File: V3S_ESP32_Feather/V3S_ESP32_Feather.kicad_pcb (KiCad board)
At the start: 4 copper layers, 30.5 x 48.3 mm, 100 parts, among them J1 USB_B_Micro, J2 Bat, J3 CAM, J4 PWM, J5 U.FL-R-SMT(01), J6 UART, J7 Micro_SD_Card_Det, J8 I2C, J9 I2C, Q1 S8050(SOT-23), U1 V3S, U2 MIC5504-1.2YM5, U3 MIC5501-3.0YM5, U4 ICM-20948, U5 ESP32-PICO-D4, U6 LT1963AxST-3.3, U7 BMP280, U8 MIC5504-1.8YM5, U9 MAX13030EEBET, Y1 X1E0000210832, Y2 CC5V-T1A 32.768KHZ +-20PPM 12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

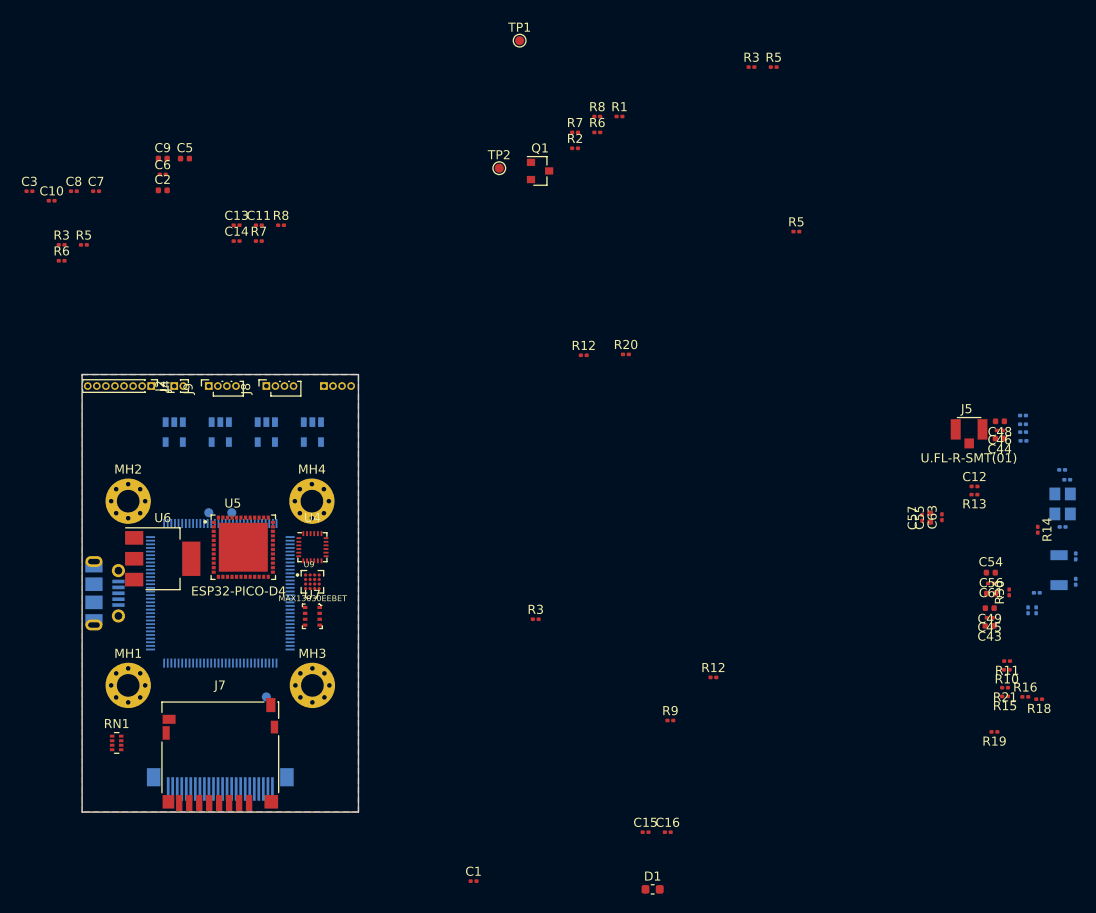
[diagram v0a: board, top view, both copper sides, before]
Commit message: New component placement, progress on rooting
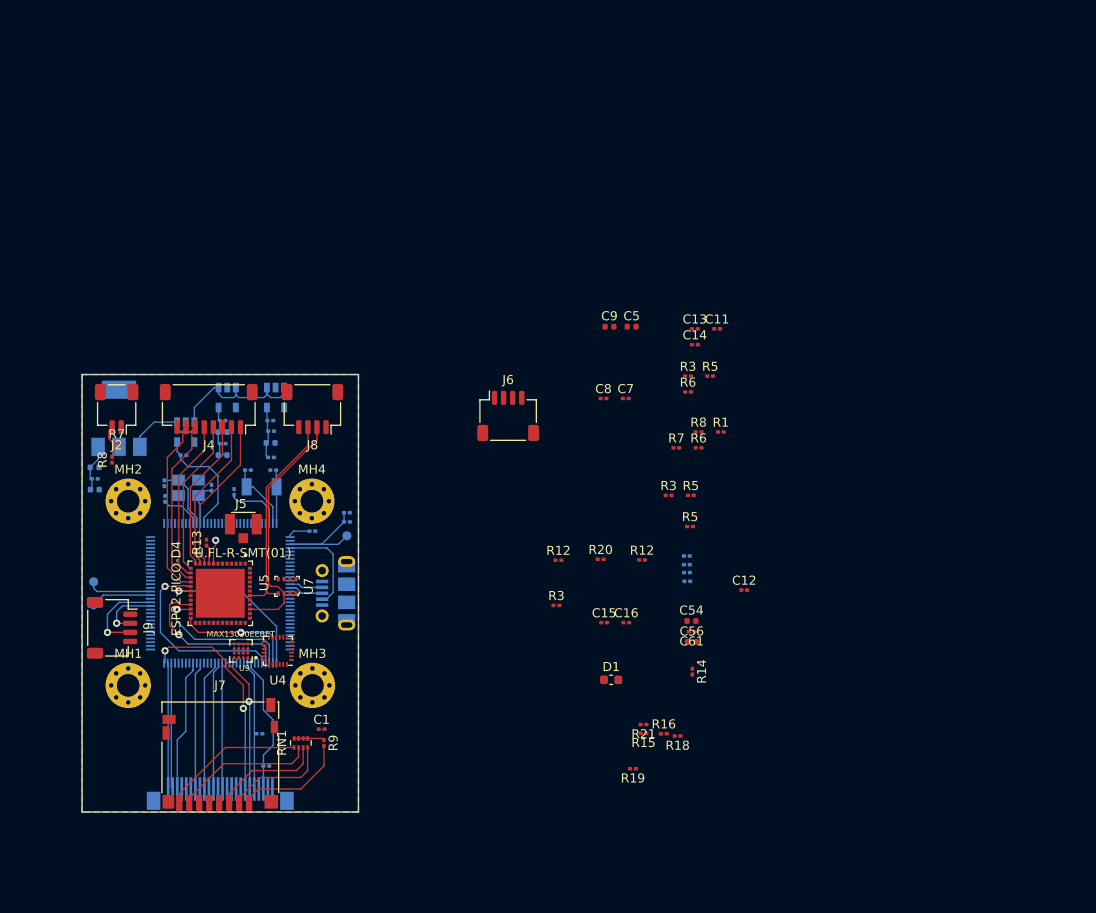
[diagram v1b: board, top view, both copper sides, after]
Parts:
- removed C2: 10uF, Capacitor_SMD:C_0402_1005Metric
- removed Q1: S8050(SOT-23), Package_TO_SOT_SMD:SOT-23
- removed R2: 100K, Resistor_SMD:R_0201_0603Metric
- removed TP1: PWR_SRC, TestPoint:TestPoint_Pad_D1.0mm
- removed the TP2 at (68.9, -2.44)
- removed the U2 at (48.3, 26.7)
- C10, C3, C43, C44, C45, C46, C48, C49, C55, C57, C6, C63, R10, R11, R30, U6: moved to B.Cu
- J2: footprint Connector_PinHeader_1.00mm:PinHeader_1x02_P1.00mm_Vertical -> Connector_JST:JST_SH_SM02B-SRSS-TB_1x02-1MP_P1.00mm_Horizontal
- J4: footprint Connector_PinHeader_1.00mm:PinHeader_1x08_P1.00mm_Vertical -> Connector_JST:JST_SH_SM08B-SRSS-TB_1x08-1MP_P1.00mm_Horizontal
- J6: footprint Connector_PinHeader_1.00mm:PinHeader_1x04_P1.00mm_Vertical -> Connector_JST:JST_SH_SM04B-SRSS-TB_1x04-1MP_P1.00mm_Horizontal; moved to F.Cu
- J8, J9: footprint Connector_PinSocket_1.00mm:PinSocket_1x04_P1.00mm_Vertical -> Connector_JST:JST_SH_SM04B-SRSS-TB_1x04-1MP_P1.00mm_Horizontal
- moved C48 100.0 mm to (24.2, 30.6), turned to 0 degrees
- moved C44 100.0 mm to (24.3, 33.0), turned to 0 degrees
- moved C46 100.0 mm to (24.3, 31.8), turned to 0 degrees
- moved C37 99.6 mm to (31.9, 32.3), turned to 270 degrees
- moved R4 99.0 mm to (32.0, 34.0), turned to 90 degrees
- moved Y1 96.4 mm to (34.6, 32.8), turned to 0 degrees
- moved C36 94.0 mm to (37.1, 32.8), turned to 90 degrees
- moved C41 91.8 mm to (41.1, 30.9), turned to 180 degrees
- moved C40 89.4 mm to (43.9, 30.9), turned to 0 degrees
- moved Y2 88.4 mm to (42.7, 32.7), turned to 270 degrees
- moved C49 86.8 mm to (38.4, 26.7), turned to 0 degrees
- moved C45 86.8 mm to (38.4, 27.9), turned to 0 degrees
- moved C43 86.7 mm to (38.4, 29.2), turned to 0 degrees
- moved R30 86.2 mm to (39.6, 33.3), turned to 270 degrees
- moved R13 84.9 mm to (36.6, 38.9), turned to 90 degrees
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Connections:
- C5 pad 1: /PMIC Power Battery/VIN -> +BATT
- D1 pad 1: /PMIC Power Battery/VIN -> +BATT
- J3 pad 1: (no net) -> /All V3s input output/STROBE
- J3 pad 10: (no net) -> Net-(J3-Pad10)
- J4 pad 1: GND -> /IO34
- J4 pad 2: /IO34 -> /IO35
- J4 pad 3: /IO33 -> /IO32
- J4 pad 4: /IO32 -> /IO33
- J4 pad 5: /IO27 -> /IO25
- J4 pad 7: /IO25 -> /IO27
- J6 pad 3: (no net) -> /TX
- J7 pad 10: (no net) -> Net-(J7-Pad10)
- J7 pad 9: (no net) -> Net-(J7-Pad9)
- R1 pad 1: VBUS -> Net-(D1-Pad2)
- R1 pad 2: Net-(D1-Pad2) -> VBUS
- RN1 pad 1: /All V3s input output/PF4 -> /All V3s input output/PF0
- RN1 pad 2: /All V3s input output/PF3 -> /All V3s input output/PF1
- RN1 pad 3: /All V3s input output/PF1 -> /All V3s input output/PF3
- RN1 pad 4: /All V3s input output/PF0 -> /All V3s input output/PF4
- U1 pad 10: (no net) -> Net-(U1-Pad10)
- U1 pad 11: (no net) -> Net-(U1-Pad11)
- U1 pad 112: (no net) -> Net-(U1-Pad112)
- U1 pad 113: (no net) -> Net-(U1-Pad113)
- U1 pad 114: (no net) -> Net-(U1-Pad114)
- U1 pad 120: (no net) -> Net-(U1-Pad120)
- U1 pad 121: (no net) -> Net-(U1-Pad121)
- U1 pad 124: (no net) -> Net-(U1-Pad124)
- U1 pad 125: (no net) -> Net-(U1-Pad125)
- U1 pad 13: (no net) -> Net-(U1-Pad13)
- U1 pad 14: (no net) -> Net-(U1-Pad14)
- U1 pad 43: (no net) -> Net-(U1-Pad43)
- U1 pad 44: (no net) -> Net-(U1-Pad44)
- U1 pad 52: (no net) -> Net-(U1-Pad52)
- U1 pad 53: (no net) -> Net-(U1-Pad53)
- U1 pad 54: (no net) -> Net-(U1-Pad54)
- U1 pad 55: (no net) -> Net-(U1-Pad55)
- U1 pad 6: (no net) -> Net-(U1-Pad6)
- U1 pad 7: (no net) -> Net-(U1-Pad7)
- U1 pad 77: (no net) -> Net-(U1-Pad77)
- U1 pad 78: (no net) -> Net-(U1-Pad78)
- U1 pad 81: (no net) -> Net-(U1-Pad81)
- U1 pad 82: (no net) -> Net-(U1-Pad82)
- U1 pad 83: (no net) -> Net-(U1-Pad83)
- U1 pad 84: (no net) -> Net-(U1-Pad84)
- U1 pad 86: (no net) -> Net-(U1-Pad86)
- U1 pad 87: (no net) -> Net-(U1-Pad87)
- U1 pad 89: (no net) -> Net-(U1-Pad89)
- U1 pad 90: (no net) -> Net-(U1-Pad90)
- U1 pad 91: (no net) -> Net-(U1-Pad91)
- U1 pad 92: (no net) -> Net-(U1-Pad92)
- U2 pad 1: /PMIC Power Battery/VIN -> +BATT
- U2 pad 3: /PMIC Power Battery/VIN -> +BATT
- U3 pad 1: /PMIC Power Battery/VIN -> +BATT
- U3 pad 3: /PMIC Power Battery/VIN -> +BATT
- U3 pad 4: (no net) -> Net-(U3-Pad4)
- U4 pad 1: (no net) -> Net-(U4-Pad1)
- U4 pad 14: (no net) -> Net-(U4-Pad14)
- U4 pad 15: (no net) -> Net-(U4-Pad15)
- U4 pad 16: (no net) -> Net-(U4-Pad16)
- U4 pad 17: (no net) -> Net-(U4-Pad17)
- U4 pad 19: (no net) -> Net-(U4-Pad19)
- U4 pad 2: (no net) -> Net-(U4-Pad2)
- U4 pad 21: (no net) -> Net-(U4-Pad21)
- U4 pad 3: (no net) -> Net-(U4-Pad3)
- U4 pad 4: (no net) -> Net-(U4-Pad4)
- U4 pad 5: (no net) -> Net-(U4-Pad5)
- U4 pad 6: (no net) -> Net-(U4-Pad6)
- U4 pad 7: (no net) -> Net-(U4-Pad7)
- U5 pad 11: (no net) -> /IO35
- U5 pad 25: (no net) -> Net-(U5-Pad25)
- U5 pad 26: (no net) -> Net-(U5-Pad26)
- U5 pad 27: (no net) -> Net-(U5-Pad27)
- U5 pad 28: (no net) -> /TX
- U5 pad 29: (no net) -> /WIFI, BT, RT/SD3
- U5 pad 30: (no net) -> Net-(U5-Pad30)
- U5 pad 31: (no net) -> Net-(U5-Pad31)
- U5 pad 32: (no net) -> Net-(U5-Pad32)
- U5 pad 33: (no net) -> Net-(U5-Pad33)
- U5 pad 5: (no net) -> Net-(U5-Pad5)
- U6 pad 1: /PMIC Power Battery/VIN -> +BATT
- U8 pad 1: /PMIC Power Battery/VIN -> +BATT
- U8 pad 3: /PMIC Power Battery/VIN -> +BATT
- U8 pad 4: (no net) -> Net-(U8-Pad4)
- U9 pad A1: (no net) -> Net-(U9-PadA1)
- U9 pad A2: (no net) -> Net-(U9-PadA2)
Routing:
- net +BATT: track 0.00 -> 30.2 mm
- net /SDA: track 0.00 -> 26.8 mm
- net /SCL: track 0.00 -> 24.3 mm
- net /All V3s input output/~CSI_RST: track 0.00 -> 24.1 mm, vias 0 -> 2
- net /All V3s input output/SDIO1_CLK: track 0.00 -> 21.2 mm, vias 0 -> 1
- net /IO27: track 0.00 -> 19.6 mm
- net /IO26: track 0.00 -> 18.8 mm
- net /All V3s input output/SDIO1_CMD: track 0.00 -> 18.1 mm, vias 0 -> 1
- net /IO25: track 0.00 -> 18.0 mm
- net /All V3s input output/SDIO1_DAT2: track 0.00 -> 17.7 mm, vias 0 -> 1
- net /IO33: track 0.00 -> 17.3 mm
- net /IO34: track 0.00 -> 17.1 mm
- net /IO35: track 0.00 -> 16.9 mm
- net /IO32: track 0.00 -> 16.7 mm
- net /All V3s input output/SDIO1_DAT0: track 0.00 -> 16.2 mm, vias 0 -> 1
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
